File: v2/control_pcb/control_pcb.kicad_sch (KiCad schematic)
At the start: 16 parts, among them J1 Raspberry_Pi_2_3, J10 8P8C_Shielded, J2 8P8C_Shielded, J6 Screw_Terminal_01x02, J7 Screw_Terminal_01x02, J8 Screw_Terminal_01x08, J9 Screw_Terminal_01x08, U3 Raspberry_Pi_Pico_2

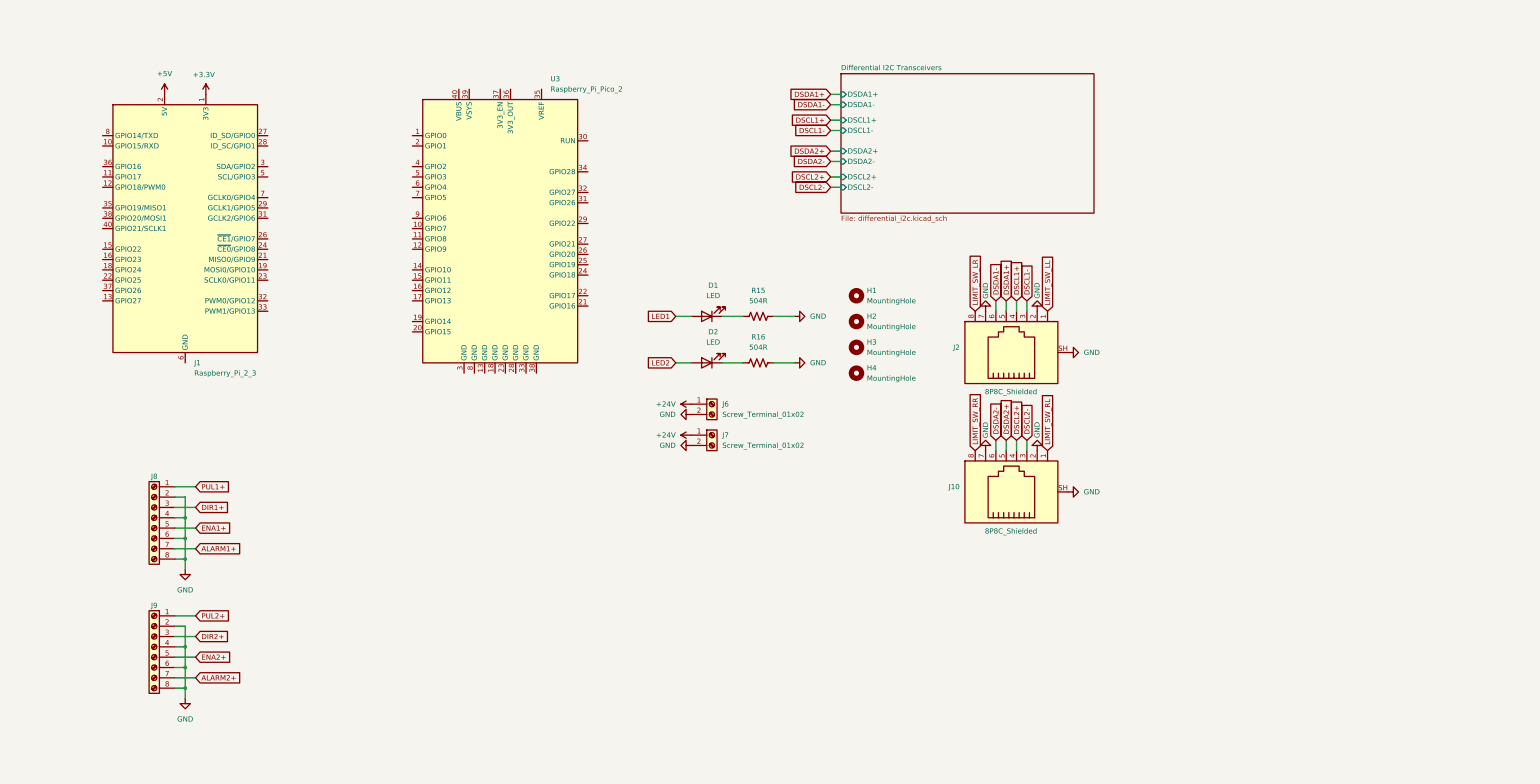
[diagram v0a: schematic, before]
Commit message: Doing stuff
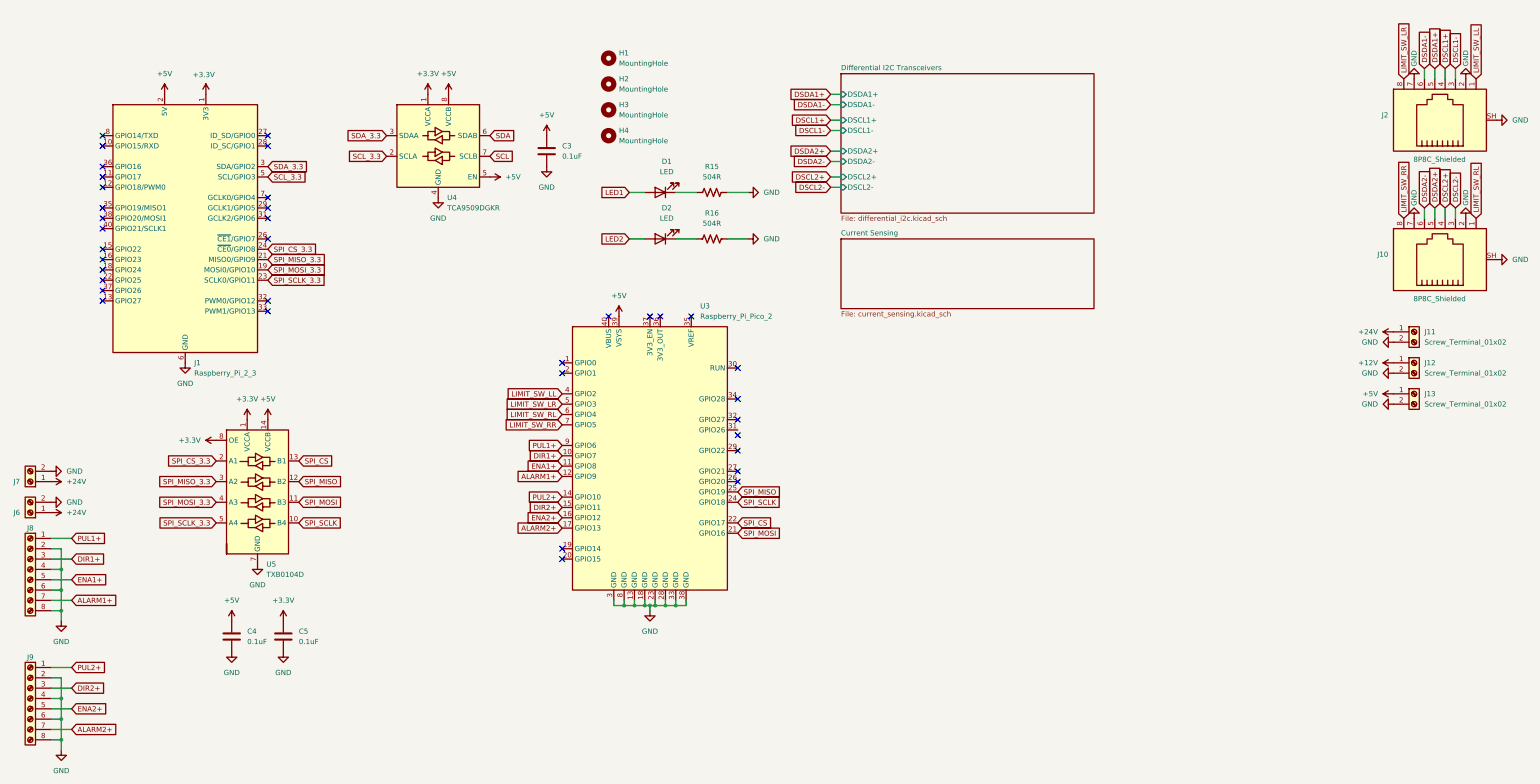
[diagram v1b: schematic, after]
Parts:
- added C3, C4, C5: 0.1uF, Capacitor_THT:C_Rect_L4.6mm_W2.0mm_P2.50mm_MKS02_FKP02, symbol Device:C
- added J11, J12, J13: Screw_Terminal_01x02, TerminalBlock_Phoenix:TerminalBlock_Phoenix_PT-1,5-2-5.0-H_1x02_P5.00mm_Horizontal, symbol Connector:Screw_Terminal_01x02
- added U4: TCA9509DGKR, Package_SO:VSSOP-8_3x3mm_P0.65mm, symbol Logic_LevelTranslator:TCA9517ADGK
- added U5: TXB0104D, Package_SO:SOIC-14_3.9x8.7mm_P1.27mm, symbol Logic_LevelTranslator:TXB0104D
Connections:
- net +24V: now also J11.1 (Pin_1)
- net +3.3V: now also C5.1, U4.1 (VCCA), U5.1 (VCCA), U5.8 (OE)
- net +5V: now also U3.39 (VSYS), C3.1, C4.1, J13.1 (Pin_1), U4.5 (EN), U4.8 (VCCB), U5.14 (VCCB)
- net ALARM1+: now also U3.12 (GPIO9)
- net ALARM2+: now also U3.17 (GPIO13)
- net DIR1+: now also U3.10 (GPIO7)
- net DIR2+: now also U3.15 (GPIO11)
- net ENA1+: now also U3.11 (GPIO8)
- net ENA2+: now also U3.16 (GPIO12)
- net GND: now also J1.14 (GND), J1.20 (GND), J1.25 (GND), J1.30 (GND), J1.34 (GND), J1.39 (GND), J1.6 (GND), J1.9 (GND), U3.13 (GND), U3.18 (GND), U3.23 (GND), U3.28 (GND), U3.3 (GND), U3.33 (GND), U3.38 (GND), U3.8 (GND), C3.2, C4.2, C5.2, J11.2 (Pin_2), J12.2 (Pin_2), J13.2 (Pin_2), U4.4 (GND), U5.7 (GND)
- net LIMIT_SW_LL: now also U3.4 (GPIO2)
- net LIMIT_SW_LR: now also U3.5 (GPIO3)
- net LIMIT_SW_RL: now also U3.6 (GPIO4)
- net LIMIT_SW_RR: now also U3.7 (GPIO5)
- net PUL1+: now also U3.9 (GPIO6)
- net PUL2+: now also U3.14 (GPIO10)
- net SPI_MOSI: now reaches U3.21 (GPIO16)
- net SPI_MOSI: now also U5.11 (B3)
- net SPI_CS: now reaches U3.22 (GPIO17)
- net SPI_CS: now also U5.13 (B1)
- net SPI_SCLK: now reaches U3.24 (GPIO18)
- net SPI_SCLK: now also U5.10 (B4)
- net SPI_MISO: now reaches U3.25 (GPIO19)
- net SPI_MISO: now also U5.12 (B2)
- net SPI_MOSI_3.3: now reaches J1.19 (MOSI0/GPIO10)
- net SPI_MOSI_3.3: now also U5.4 (A3)
- net SPI_MISO_3.3: now reaches J1.21 (MISO0/GPIO9)
- net SPI_MISO_3.3: now also U5.3 (A2)
- net SPI_SCLK_3.3: now reaches J1.23 (SCLK0/GPIO11)
- net SPI_SCLK_3.3: now also U5.5 (A4)
- net SPI_CS_3.3: now reaches J1.24 (~{CE0}/GPIO8)
- net SPI_CS_3.3: now also U5.2 (A1)
- net SDA_3.3: now reaches J1.3 (SDA/GPIO2)
- net SDA_3.3: now also U4.3 (SDAA)
- net SCL_3.3: now reaches J1.5 (SCL/GPIO3)
- net SCL_3.3: now also U4.2 (SCLA)
- new net +12V: J12.1 (Pin_1)
- new net SCL: U4.7 (SCLB)
- new net SDA: U4.6 (SDAB)
- no-connect marks 0 -> 37
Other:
- added sheet Current Sensing (current_sensing.kicad_sch)
- moved on the sheet: D1, D2, H1, H2, H3, H4, J10, J2, J6, J7, J8, J9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
